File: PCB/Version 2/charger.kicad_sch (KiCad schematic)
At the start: 17 parts, among them U2 BQ24073RGTR, U5 WL9003S5-33

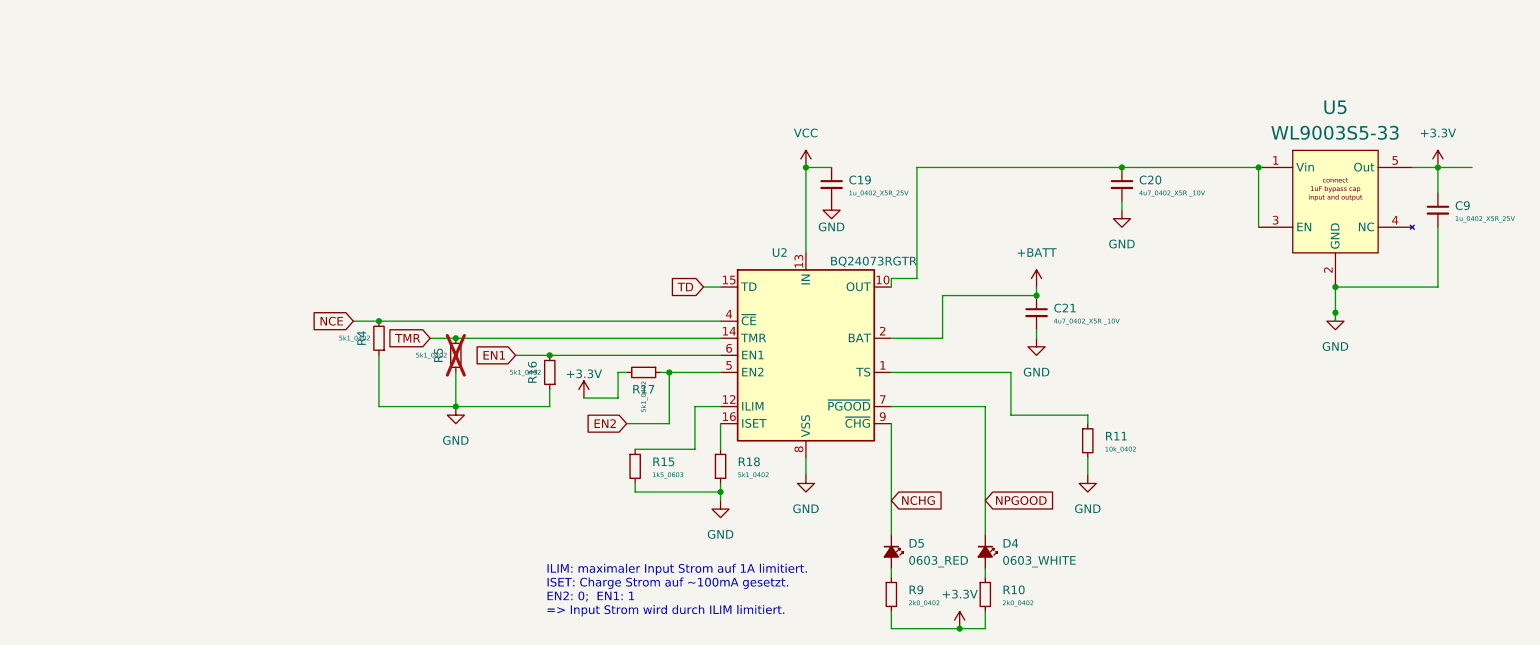
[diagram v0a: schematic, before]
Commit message: Working on Version 2
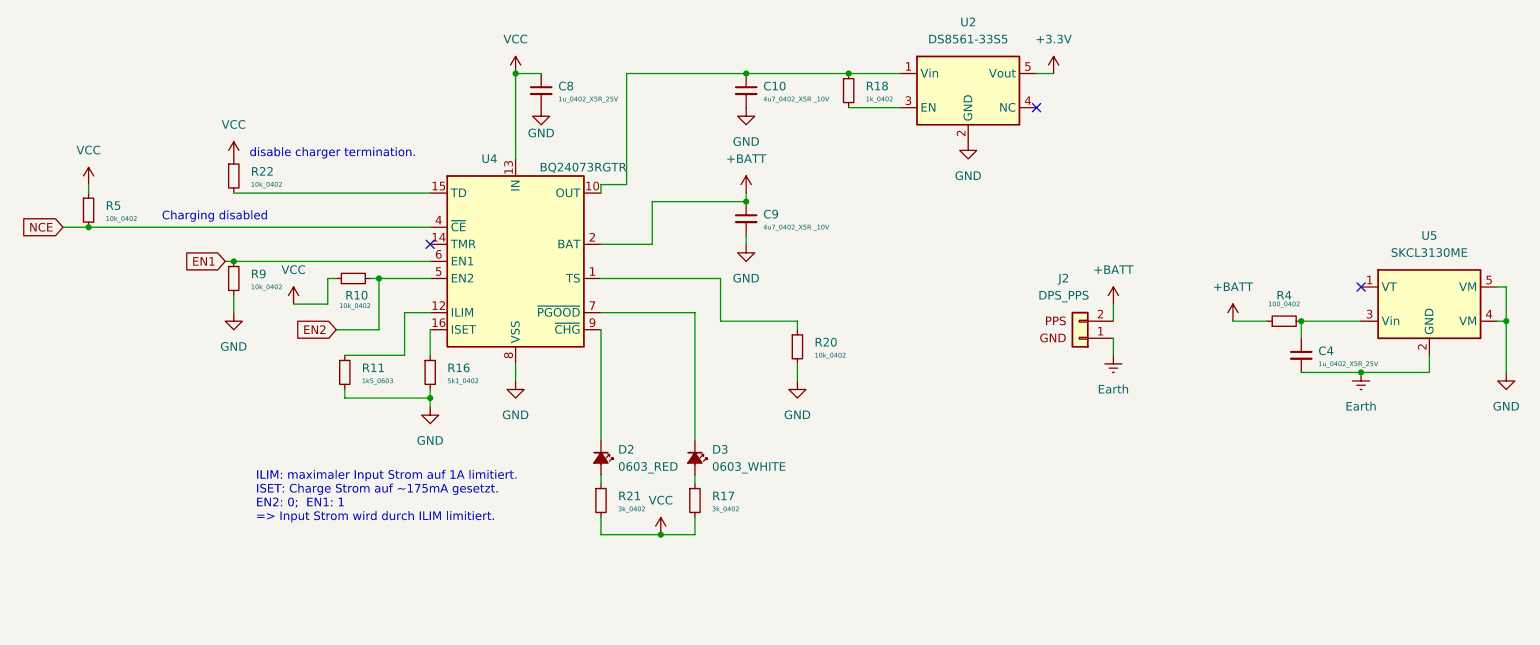
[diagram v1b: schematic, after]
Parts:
- removed C19, C9: 1u_0402_X5R_25V, Capacitor_SMD:C_0402_1005Metric, symbol capacitor_smd_standard:1u_0402_X5R_25V
- removed C20, C21: 4u7_0402_X5R _10V, Capacitor_SMD:C_0402_1005Metric, symbol capacitor_smd_extended:4u7_0402_X5R _10V
- removed D4: 0603_WHITE, LED_SMD:LED_0603_1608Metric, symbol led:0603_GREEN
- removed D5: 0603_RED, LED_SMD:LED_0603_1608Metric, symbol led:0603_RED
- removed R10, R9: 2k0_0402, Resistor_SMD:R_0402_1005Metric, symbol resistor_smd_standard:2k0_0402
- removed R11: 10k_0402, Resistor_SMD:R_0402_1005Metric, symbol resistor_smd_standard:10k_0402
- removed R15: 1k5_0603, Resistor_SMD:R_0603_1608Metric, symbol resistor_smd_standard:1k5_0603
- removed R16, R17, R4, R5: 5k1_0402, Resistor_SMD:R_0402_1005Metric, symbol resistor_smd_standard:5k1_0402
- removed R18: 5k1_0402, Resistor_SMD:R_0402_1005Metric, symbol resistor_smd_standard:8k2_0402
- removed U2: BQ24073RGTR, Package_DFN_QFN:VQFN-16-1EP_3x3mm_P0.5mm_EP1.6x1.6mm, symbol Battery_Management:BQ24072RGT
- removed U5: WL9003S5-33, Package_TO_SOT_SMD:SOT-23-5, symbol dcdc:WL9003S5-33
- added C10, C9: 4u7_0402_X5R _10V, Capacitor_SMD:C_0402_1005Metric, symbol capacitor_smd_extended:4u7_0402_X5R _10V
- added C4, C8: 1u_0402_X5R_25V, Capacitor_SMD:C_0402_1005Metric, symbol capacitor_smd_standard:1u_0402_X5R_25V
- added D2: 0603_RED, LED_SMD:LED_0603_1608Metric, symbol led:0603_RED
- added D3: 0603_WHITE, LED_SMD:LED_0603_1608Metric, symbol led:0603_GREEN
- added J2: DPS_PPS, Connector_JST:JST_PH_B2B-PH-K_1x02_P2.00mm_Vertical, symbol DPS_connectors:DPS_PPS
- added R10, R20, R22, R5, R9: 10k_0402, Resistor_SMD:R_0402_1005Metric, symbol resistor_smd_standard:10k_0402
- added R11: 1k5_0603, Resistor_SMD:R_0603_1608Metric, symbol resistor_smd_standard:1k5_0603
- added R16: 5k1_0402, Resistor_SMD:R_0402_1005Metric, symbol resistor_smd_standard:8k2_0402
- added R17, R21: 3k_0402, Resistor_SMD:R_0402_1005Metric, symbol resistor_smd_standard:3k_0402
- added R18: 1k_0402, Resistor_SMD:R_0402_1005Metric, symbol resistor_smd_standard:1k_0402
- added R4: 100_0402, Resistor_SMD:R_0402_1005Metric, symbol resistor_smd_standard:100_0402
- added U2: DS8561-33S5, Package_TO_SOT_SMD:SOT-23-5, symbol Lil-Lib:DS8561-33S5
- added U4: BQ24073RGTR, Package_DFN_QFN:VQFN-16-1EP_3x3mm_P0.5mm_EP1.6x1.6mm, symbol Battery_Management:BQ24072RGT
- added U5: SKCL3130ME, Package_TO_SOT_SMD:SOT-23-5, symbol Lil-Lib:SKCL3130ME
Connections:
- net +3.3V: now also U2.5 (Vout)
- net +BATT: now also C9.1, J2.2 (Pin_2), R4.1, U4.2 (BAT), U4.3 (BAT)
- net EN1: now also R9.1, U4.6 (EN1)
- net EN2: now also R10.2, U4.5 (EN2)
- net GND: now also C10.2, C8.2, C9.2, R11.2, R16.2, R20.2, R9.2, U2.2 (GND), U4.17 (VSS), U4.8 (VSS), U5.4 (VM), U5.5 (VM)
- net NCE: now also R5.2, U4.4 (~{CE})
- net VCC: now also C8.1, R10.1, R17.2, R21.2, R22.1, R5.1, U4.13 (IN)
- new net: D2.1 (K), U4.9 (~{CHG})
- new net: D2.2 (A), R21.1
- new net: R16.1, U4.16 (ISET)
- new net: C4.1, R4.2, U5.3 (Vin)
- new net: C10.1, R18.1, U2.1 (Vin), U4.10 (OUT), U4.11 (OUT)
- new net: R18.2, U2.3 (EN)
- new net: R11.1, U4.12 (ILIM)
- new net: R20.1, U4.1 (TS)
- new net: D3.1 (K), U4.7 (~{PGOOD})
- new net: D3.2 (A), R17.1
- new net: R22.2, U4.15 (TD)
- new net Earth: C4.2, J2.1 (Pin_1), U5.2 (GND)
- no-connect marks 0 -> 3
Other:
- note added: "Charging disabled"
- note added: "ILIM: maximaler Input Strom auf 1A limitiert. ISET: Charge Strom auf ~175mA gesetzt. EN2: 0; EN1: 1 => Input Strom wird durch ILIM limitiert."
- note added: "disable charger termination."
- note removed: "ILIM: maximaler Input Strom auf 1A limitiert. ISET: Charge Strom auf ~100mA gesetzt. EN2: 0; EN1: 1 => Input Strom wird durch ILIM limitiert."
